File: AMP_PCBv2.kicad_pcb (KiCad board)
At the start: 2 copper layers, 2 parts, among them U1 Teensy4.0, U2 Logo

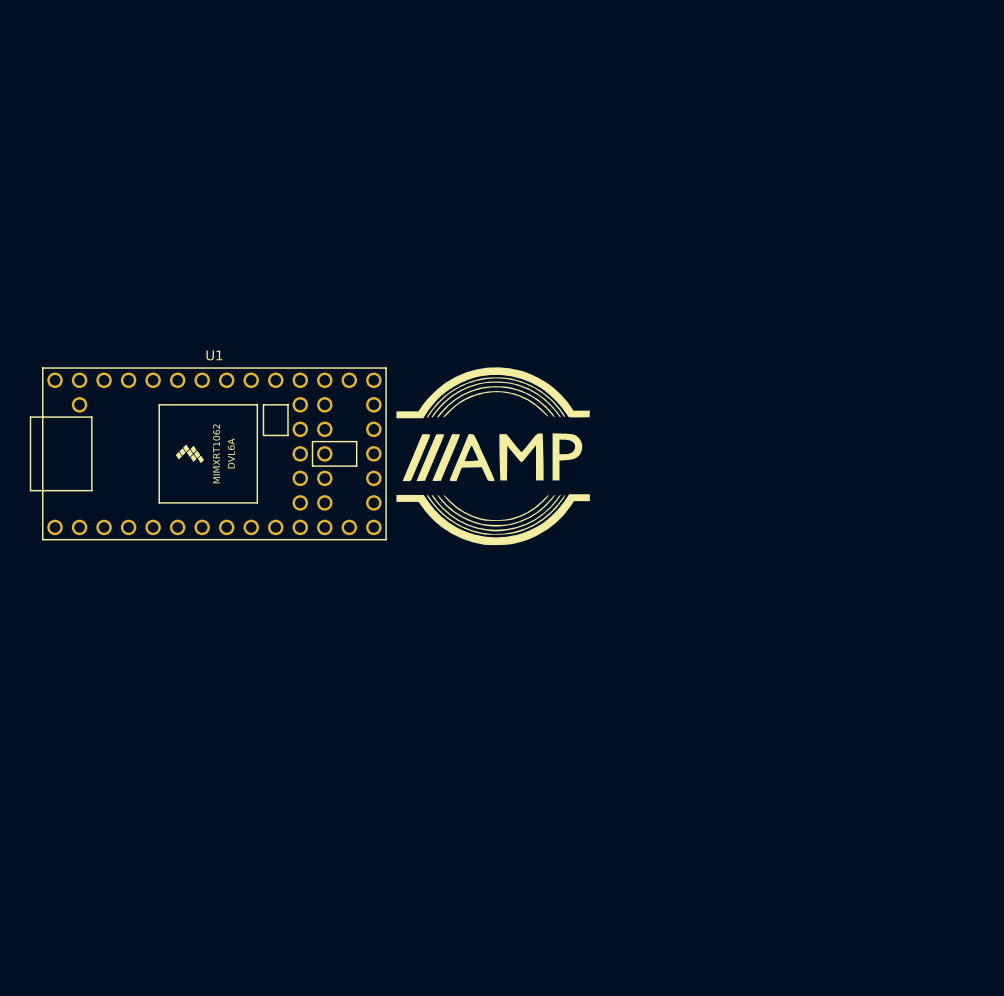
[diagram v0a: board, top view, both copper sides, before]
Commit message: Route PCB
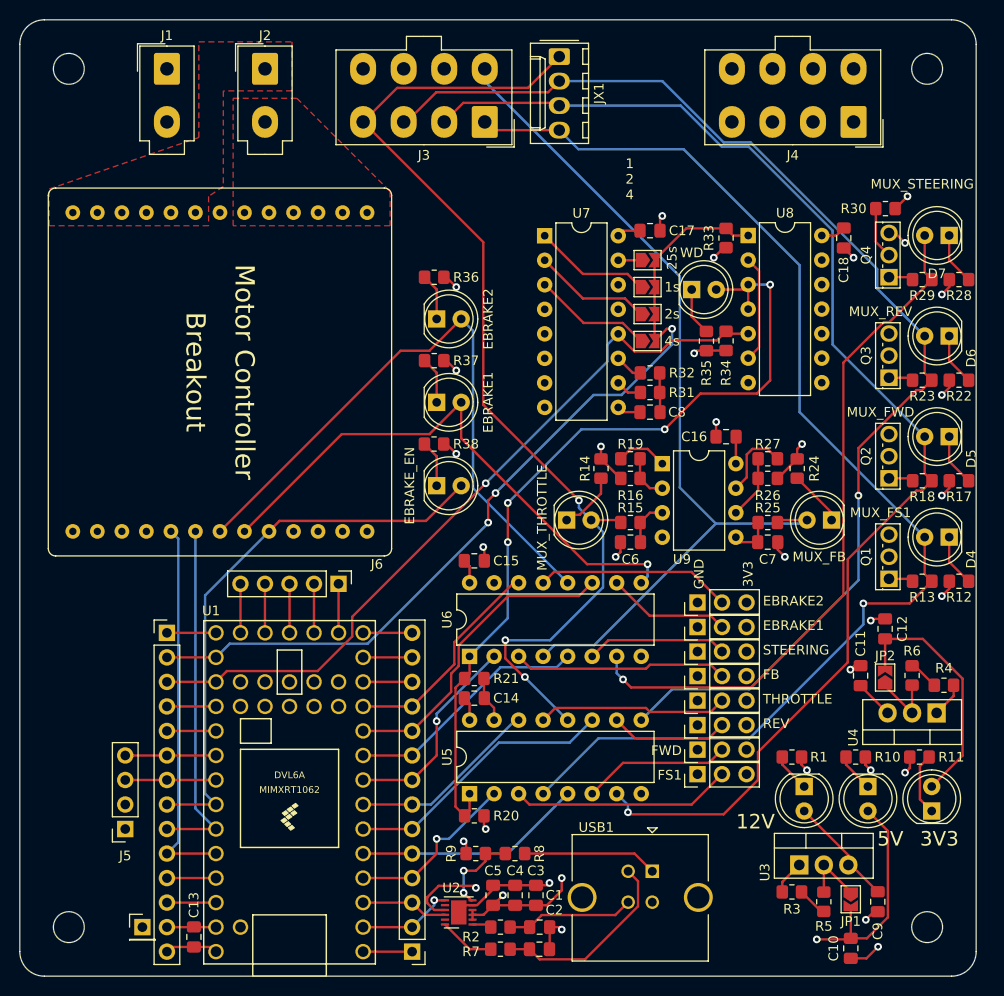
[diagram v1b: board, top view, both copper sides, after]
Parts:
- added C1: 47pF, Capacitor_SMD:C_0805_2012Metric_Pad1.18x1.45mm_HandSolder, F.Cu at (145.3, 134.6)
- added C10: 0.1uF, Capacitor_SMD:C_0805_2012Metric_Pad1.18x1.45mm_HandSolder, F.Cu at (177.5, 136.8)
- added C11: 0.1uF, Capacitor_SMD:C_0805_2012Metric_Pad1.18x1.45mm_HandSolder, F.Cu at (178.5, 108.6)
- added C12: 0.1uF, Capacitor_SMD:C_0805_2012Metric_Pad1.18x1.45mm_HandSolder, F.Cu at (181.1, 103.7)
- added C13: 0.1uF, Capacitor_SMD:C_0805_2012Metric_Pad1.18x1.45mm_HandSolder, F.Cu at (109.5, 135.6)
- added C14: 0.1uF, Capacitor_SMD:C_0805_2012Metric_Pad1.18x1.45mm_HandSolder, F.Cu at (138.5, 110.9)
- added C15: 0.1uF, Capacitor_SMD:C_0805_2012Metric_Pad1.18x1.45mm_HandSolder, F.Cu at (138.5, 96.7)
- added C16: 0.1uF, Capacitor_SMD:C_0805_2012Metric_Pad1.18x1.45mm_HandSolder, F.Cu at (164.6, 83.8)
- added C17: 0.1uF, Capacitor_SMD:C_0805_2012Metric_Pad1.18x1.45mm_HandSolder, F.Cu at (156.7, 62.5)
- added C18: 0.1uF, Capacitor_SMD:C_0805_2012Metric_Pad1.18x1.45mm_HandSolder, F.Cu at (176.8, 63.2)
- added C2: 47pF, Capacitor_SMD:C_0805_2012Metric_Pad1.18x1.45mm_HandSolder, F.Cu at (145.3, 136.9)
- added C3: 4.7uF, Capacitor_SMD:C_0805_2012Metric_Pad1.18x1.45mm_HandSolder, F.Cu at (144.9, 131.3)
- added C4: 100nF, Capacitor_SMD:C_0805_2012Metric_Pad1.18x1.45mm_HandSolder, F.Cu at (142.7, 131.3)
- added C5: 100nF, Capacitor_SMD:C_0805_2012Metric_Pad1.18x1.45mm_HandSolder, F.Cu at (140.5, 131.3)
- added C6: 10uF, Capacitor_SMD:C_0805_2012Metric_Pad1.18x1.45mm_HandSolder, F.Cu at (154.7, 94.7)
- added C7: 10uF, Capacitor_SMD:C_0805_2012Metric_Pad1.18x1.45mm_HandSolder, F.Cu at (168.9, 94.7)
- added C8: 10nF, Capacitor_SMD:C_0805_2012Metric_Pad1.18x1.45mm_HandSolder, F.Cu at (156.7, 81.3)
- added C9: 0.1uF, Capacitor_SMD:C_0805_2012Metric_Pad1.18x1.45mm_HandSolder, F.Cu at (180.3, 132.0)
- added D1: GN, LED_THT:LED_D5.0mm, F.Cu at (172.7, 120.1)
- added D10: YL, LED_THT:LED_D5.0mm, F.Cu at (134.6, 88.9)
- added D11: RD, LED_THT:LED_D5.0mm, F.Cu at (134.6, 80.3)
- added D12: RD, LED_THT:LED_D5.0mm, F.Cu at (134.6, 71.6)
- added D13: RD, LED_THT:LED_D5.0mm, F.Cu at (161.0, 68.6)
- added D2: GN, LED_THT:LED_D5.0mm, F.Cu at (179.3, 120.1)
- added D3: GN, LED_THT:LED_D5.0mm, F.Cu at (185.9, 122.6)
- added D4: YL, LED_THT:LED_D5.0mm, F.Cu at (187.7, 94.2)
- added D5: YL, LED_THT:LED_D5.0mm, F.Cu at (187.7, 83.8)
- added D6: YL, LED_THT:LED_D5.0mm, F.Cu at (187.7, 73.4)
- added D7: YL, LED_THT:LED_D5.0mm, F.Cu at (187.7, 63.0)
- added D8: YL, LED_THT:LED_D5.0mm, F.Cu at (148.1, 92.5)
- added D9: YL, LED_THT:LED_D5.0mm, F.Cu at (175.5, 92.5)
- added J1: POWER, Connector_Molex:Molex_Mini-Fit_Jr_5566-02A_2x01_P4.20mm_Vertical, F.Cu at (106.7, 45.7)
- added J2: EBRAKE, Connector_Molex:Molex_Mini-Fit_Jr_5566-02A_2x01_P4.20mm_Vertical, F.Cu at (116.8, 45.7)
- added J3: MC, Connector_Molex:Molex_Mini-Fit_Jr_5566-08A_2x04_P4.20mm_Vertical, F.Cu at (139.6, 51.2)
- added J4: STEERING, Connector_Molex:Molex_Mini-Fit_Jr_5566-08A_2x04_P4.20mm_Vertical, F.Cu at (177.8, 51.2)
- added J5: OLED Breakout, Connector_PinSocket_2.54mm:PinSocket_1x04_P2.54mm_Vertical, F.Cu at (102.4, 124.5)
- added J6: EBRAKE_BREAKOUT, AMP:AMP_Brake_Controller_Breakout, F.Cu at (130.0, 96.2)
- added JP1: 5VOB, Jumper:SolderJumper-2_P1.3mm_Open_TrianglePad1.0x1.5mm, F.Cu at (177.5, 131.7)
- added JP10: Jumper_EBRAKE2, Connector_PinHeader_2.54mm:PinHeader_1x03_P2.54mm_Vertical, F.Cu at (161.6, 101.0)
- added JP11: 0.25s, Jumper:SolderJumper-2_P1.3mm_Open_TrianglePad1.0x1.5mm, F.Cu at (156.5, 65.5)
- added JP12: 1s, Jumper:SolderJumper-2_P1.3mm_Open_TrianglePad1.0x1.5mm, F.Cu at (156.5, 68.3)
- added JP13: 2s, Jumper:SolderJumper-2_P1.3mm_Open_TrianglePad1.0x1.5mm, F.Cu at (156.5, 71.1)
- added JP14: 4s, Jumper:SolderJumper-2_P1.3mm_Open_TrianglePad1.0x1.5mm, F.Cu at (156.5, 73.9)
- added JP2: 3V3OB, Jumper:SolderJumper-2_P1.3mm_Open_TrianglePad1.0x1.5mm, F.Cu at (181.1, 108.8)
- added JP3: Jumper_FS1, Connector_PinHeader_2.54mm:PinHeader_1x03_P2.54mm_Vertical, F.Cu at (161.6, 118.8)
- added JP4: Jumper_FWD, Connector_PinHeader_2.54mm:PinHeader_1x03_P2.54mm_Vertical, F.Cu at (161.6, 116.2)
- added JP5: Jumper_REV, Connector_PinHeader_2.54mm:PinHeader_1x03_P2.54mm_Vertical, F.Cu at (161.6, 113.7)
- added JP6: Jumper_THROTTLE, Connector_PinHeader_2.54mm:PinHeader_1x03_P2.54mm_Vertical, F.Cu at (161.6, 111.2)
- added JP7: Jumper_RB, Connector_PinHeader_2.54mm:PinHeader_1x03_P2.54mm_Vertical, F.Cu at (161.6, 108.6)
- added JP8: Jumper_STEERING, Connector_PinHeader_2.54mm:PinHeader_1x03_P2.54mm_Vertical, F.Cu at (161.6, 106.1)
- added JP9: Jumper_EBRAKE1, Connector_PinHeader_2.54mm:PinHeader_1x03_P2.54mm_Vertical, F.Cu at (161.6, 103.5)
- added JT1: Conn_01x14_Male, Connector_PinHeader_2.54mm:PinHeader_1x14_P2.54mm_Vertical, F.Cu at (132.1, 137.2)
- added JT2: Conn_01x05_Male, Connector_PinHeader_2.54mm:PinHeader_1x05_P2.54mm_Vertical, F.Cu at (124.5, 99.1)
- added JT3: Conn_01x14_Male, Connector_PinHeader_2.54mm:PinHeader_1x14_P2.54mm_Vertical, F.Cu at (106.7, 104.1)
- added JT4: Conn_01x01_Male, Connector_PinHeader_2.54mm:PinHeader_1x01_P2.54mm_Vertical, F.Cu at (104.1, 134.6)
- added JX1: MC_OLD, Connector_Molex:Molex_KK-254_AE-6410-04A_1x04_P2.54mm_Vertical, F.Cu at (147.3, 44.5)
- added Q1: Q_NMOS_GDS, Package_TO_SOT_THT:TO-251-3_Vertical, F.Cu at (181.5, 98.5)
- added Q2: Q_NMOS_GDS, Package_TO_SOT_THT:TO-251-3_Vertical, F.Cu at (181.5, 88.1)
- added Q3: Q_NMOS_GDS, Package_TO_SOT_THT:TO-251-3_Vertical, F.Cu at (181.5, 77.7)
- added Q4: Q_NMOS_GDS, Package_TO_SOT_THT:TO-251-3_Vertical, F.Cu at (181.5, 67.3)
- added R1: 560, Resistor_SMD:R_0805_2012Metric_Pad1.20x1.40mm_HandSolder, F.Cu at (171.4, 117.0)
- added R10: 130, Resistor_SMD:R_0805_2012Metric_Pad1.20x1.40mm_HandSolder, F.Cu at (178.0, 117.0)
- added R11: 56, Resistor_SMD:R_0805_2012Metric_Pad1.20x1.40mm_HandSolder, F.Cu at (184.6, 117.0)
- added R12: 56, Resistor_SMD:R_0805_2012Metric_Pad1.20x1.40mm_HandSolder, F.Cu at (188.7, 98.8)
- added R13: 1K, Resistor_SMD:R_0805_2012Metric_Pad1.20x1.40mm_HandSolder, F.Cu at (184.9, 98.8)
- added R14: 56, Resistor_SMD:R_0805_2012Metric_Pad1.20x1.40mm_HandSolder, F.Cu at (151.6, 87.1)
- added R15: 1K, Resistor_SMD:R_0805_2012Metric_Pad1.20x1.40mm_HandSolder, F.Cu at (154.7, 92.7)
- added R16: 1K, Resistor_SMD:R_0805_2012Metric_Pad1.20x1.40mm_HandSolder, F.Cu at (154.7, 88.1)
- added R17: 56, Resistor_SMD:R_0805_2012Metric_Pad1.20x1.40mm_HandSolder, F.Cu at (188.7, 88.4)
- added R18: 1K, Resistor_SMD:R_0805_2012Metric_Pad1.20x1.40mm_HandSolder, F.Cu at (184.9, 88.4)
- added R19: 1.8K, Resistor_SMD:R_0805_2012Metric_Pad1.20x1.40mm_HandSolder, F.Cu at (154.7, 86.1)
- added R2: 27, Resistor_SMD:R_0805_2012Metric_Pad1.20x1.40mm_HandSolder, F.Cu at (141.2, 134.6)
- added R20: 10K, Resistor_SMD:R_0805_2012Metric_Pad1.20x1.40mm_HandSolder, F.Cu at (138.5, 123.1)
- added R21: 10K, Resistor_SMD:R_0805_2012Metric_Pad1.20x1.40mm_HandSolder, F.Cu at (138.5, 108.9)
- added R22: 56, Resistor_SMD:R_0805_2012Metric_Pad1.20x1.40mm_HandSolder, F.Cu at (188.7, 78.0)
- added R23: 1K, Resistor_SMD:R_0805_2012Metric_Pad1.20x1.40mm_HandSolder, F.Cu at (184.9, 78.0)
- added R24: 56, Resistor_SMD:R_0805_2012Metric_Pad1.20x1.40mm_HandSolder, F.Cu at (172.0, 87.1)
- added R25: 1K, Resistor_SMD:R_0805_2012Metric_Pad1.20x1.40mm_HandSolder, F.Cu at (168.9, 92.7)
- added R26: 1K, Resistor_SMD:R_0805_2012Metric_Pad1.20x1.40mm_HandSolder, F.Cu at (168.9, 88.1)
- added R27: 1.8K, Resistor_SMD:R_0805_2012Metric_Pad1.20x1.40mm_HandSolder, F.Cu at (168.9, 86.1)
- added R28: 56, Resistor_SMD:R_0805_2012Metric_Pad1.20x1.40mm_HandSolder, F.Cu at (188.7, 67.5)
- added R29: 1K, Resistor_SMD:R_0805_2012Metric_Pad1.20x1.40mm_HandSolder, F.Cu at (184.9, 67.5)
- added R3: 10K, Resistor_SMD:R_0805_2012Metric_Pad1.20x1.40mm_HandSolder, F.Cu at (171.4, 131.0)
- added R30: 1K, Resistor_SMD:R_0805_2012Metric_Pad1.20x1.40mm_HandSolder, F.Cu at (181.1, 60.2)
- added R31: 15K, Resistor_SMD:R_0805_2012Metric_Pad1.20x1.40mm_HandSolder, F.Cu at (156.7, 79.2)
- added R32: 6.2K, Resistor_SMD:R_0805_2012Metric_Pad1.20x1.40mm_HandSolder, F.Cu at (156.7, 77.2)
- added R33: 10K, Resistor_SMD:R_0805_2012Metric_Pad1.20x1.40mm_HandSolder, F.Cu at (164.6, 63.2)
- added R34: 10K, Resistor_SMD:R_0805_2012Metric_Pad1.20x1.40mm_HandSolder, F.Cu at (164.6, 73.9)
- added R35: 33, Resistor_SMD:R_0805_2012Metric_Pad1.20x1.40mm_HandSolder, F.Cu at (162.6, 73.9)
- added R36: 33, Resistor_SMD:R_0805_2012Metric_Pad1.20x1.40mm_HandSolder, F.Cu at (134.4, 67.3)
- added R37: 33, Resistor_SMD:R_0805_2012Metric_Pad1.20x1.40mm_HandSolder, F.Cu at (134.4, 75.9)
- added R38: 56, Resistor_SMD:R_0805_2012Metric_Pad1.20x1.40mm_HandSolder, F.Cu at (134.3, 84.6)
- added R4: 10K, Resistor_SMD:R_0805_2012Metric_Pad1.20x1.40mm_HandSolder, F.Cu at (187.2, 109.6)
- added R5: 3.3K, Resistor_SMD:R_0805_2012Metric_Pad1.20x1.40mm_HandSolder, F.Cu at (174.7, 132.0)
- added R6: 6.2K, Resistor_SMD:R_0805_2012Metric_Pad1.20x1.40mm_HandSolder, F.Cu at (183.9, 108.6)
- added R7: 27, Resistor_SMD:R_0805_2012Metric_Pad1.20x1.40mm_HandSolder, F.Cu at (141.2, 136.9)
- added R8: 4.7K, Resistor_SMD:R_0805_2012Metric_Pad1.20x1.40mm_HandSolder, F.Cu at (142.7, 127.0)
- added R9: 10K, Resistor_SMD:R_0805_2012Metric_Pad1.20x1.40mm_HandSolder, F.Cu at (138.7, 127.0)
- added REF**: MountingHole_3.2mm_M3, MountingHole:MountingHole_3.2mm_M3, F.Cu at (96.5, 45.7)
- added REF**: MountingHole_3.2mm_M3, MountingHole:MountingHole_3.2mm_M3, F.Cu at (96.5, 134.6)
- added REF**: MountingHole_3.2mm_M3, MountingHole:MountingHole_3.2mm_M3, F.Cu at (185.4, 45.7)
- added REF**: MountingHole_3.2mm_M3, MountingHole:MountingHole_3.2mm_M3, F.Cu at (185.4, 134.6)
- added U3: LM1117-ADJ, Package_TO_SOT_THT:TO-220-3_Vertical, F.Cu at (172.2, 128.2)
- added U4: LM1117-ADJ, Package_TO_SOT_THT:TO-220-3_Vertical, F.Cu at (186.4, 112.4)
- added U5: 74HC157, Package_DIP:DIP-16_W7.62mm, F.Cu at (138.0, 120.8)
- added U6: 74HC157, Package_DIP:DIP-16_W7.62mm, F.Cu at (138.0, 106.6)
- added U7: 74HC4060, Package_DIP:DIP-16_W7.62mm, F.Cu at (145.8, 63.0)
- added U8: 74HC00, Package_DIP:DIP-14_W7.62mm, F.Cu at (166.9, 63.0)
- added U9: TLV272, Package_DIP:DIP-8_W7.62mm, F.Cu at (158.0, 86.6)
- added USB1: USB_B, Connector_USB:USB_B_TE_5787834_Vertical, F.Cu at (157.0, 128.8)
- U2: value Logo -> FT234XD; footprint AMP:Logo -> Package_DFN_QFN:DFN-12-1EP_3x3mm_P0.5mm_EP1.6x2.5mm
- moved U2 47.2 mm to (136.9, 133.1), turned to 180 degrees
- moved U1 35.9 mm to (119.4, 120.7), turned to 90 degrees
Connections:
- U1 pad 1: unconnected-(U1-Pad1) -> GND
- U1 pad 10: unconnected-(U1-Pad10) -> /MCU_EBRAKE1
- U1 pad 11: unconnected-(U1-Pad11) -> /MCU_EBRAKE2
- U1 pad 12: unconnected-(U1-Pad12) -> Net-(U1-Pad12)
- U1 pad 13: unconnected-(U1-Pad13) -> Net-(U1-Pad13)
- U1 pad 14: unconnected-(U1-Pad14) -> Net-(U1-Pad14)
- U1 pad 15: unconnected-(U1-Pad15) -> Net-(U1-Pad15)
- U1 pad 16: unconnected-(U1-Pad16) -> Net-(U1-Pad16)
- U1 pad 17: unconnected-(U1-Pad17) -> GND
- U1 pad 18: unconnected-(U1-Pad18) -> Net-(U1-Pad18)
- U1 pad 19: unconnected-(U1-Pad19) -> Net-(U1-Pad19)
- U1 pad 2: unconnected-(U1-Pad2) -> /RX1
- U1 pad 20: unconnected-(U1-Pad20) -> Net-(U1-Pad20)
- U1 pad 21: unconnected-(U1-Pad21) -> /WD_SET
- U1 pad 22: unconnected-(U1-Pad22) -> /WD_RESET
- U1 pad 23: unconnected-(U1-Pad23) -> Net-(U1-Pad23)
- U1 pad 24: unconnected-(U1-Pad24) -> Net-(U1-Pad24)
- U1 pad 25: unconnected-(U1-Pad25) -> /OLED_SDA
- U1 pad 26: unconnected-(U1-Pad26) -> /OLED_SCL
- U1 pad 27: unconnected-(U1-Pad27) -> /EBRAKE_EN
- U1 pad 28: unconnected-(U1-Pad28) -> /EBRAKE_IS1
- U1 pad 29: unconnected-(U1-Pad29) -> /EBRAKE_IS2
- U1 pad 3: unconnected-(U1-Pad3) -> /TX1
- U1 pad 30: unconnected-(U1-Pad30) -> Net-(U1-Pad30)
- U1 pad 31: unconnected-(U1-Pad31) -> Net-(U1-Pad31)
- U1 pad 32: unconnected-(U1-Pad32) -> GND
- U1 pad 33: unconnected-(U1-Pad33) -> +5V
- U1 pad 34: unconnected-(U1-Pad34) -> Net-(U1-Pad34)
- U1 pad 4: unconnected-(U1-Pad4) -> /MCU_FS1
- U1 pad 5: unconnected-(U1-Pad5) -> /MCU_FWD
- U1 pad 6: unconnected-(U1-Pad6) -> /MCU_REV
- U1 pad 7: unconnected-(U1-Pad7) -> /MCU_THROTTLE
- U1 pad 8: unconnected-(U1-Pad8) -> /MCU_FB
- U1 pad 9: unconnected-(U1-Pad9) -> /MCU_STEERING
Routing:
- net +5V: track 0.00 -> 201.0 mm, vias 0 -> 1
- net /MUX_FWD: track 0.00 -> 132.9 mm, vias 0 -> 1
- net /MUX_FS1: track 0.00 -> 127.8 mm, vias 0 -> 1
- net /MUX_REV: track 0.00 -> 125.4 mm, vias 0 -> 1
- net +3V3: track 0.00 -> 115.2 mm, vias 0 -> 3
- net /MUX_THROTTLE: track 0.00 -> 108.2 mm, vias 0 -> 3
- net GND: track 0.00 -> 95.4 mm, vias 0 -> 29
- net /MUX_FB: track 0.00 -> 93.4 mm
- net /WD_SET: track 0.00 -> 90.8 mm, vias 0 -> 3
- net /WD_SEL: track 0.00 -> 88.3 mm, vias 0 -> 4
- net /WD_RESET: track 0.00 -> 79.2 mm, vias 0 -> 1
- net /MUX_STEERING: track 0.00 -> 71.5 mm, vias 0 -> 1
- net /MUX_EBRAKE2: track 0.00 -> 66.0 mm
- net /MUX_EBRAKE1: track 0.00 -> 58.6 mm, vias 0 -> 1
- net /EBRAKE_EN: track 0.00 -> 58.4 mm
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- added copper zone on In1.Cu, net +12V
- added copper zone on F.Cu, net /OUT_EBRAKE1
- added copper zone on F.Cu, net /OUT_EBRAKE2
- added copper zone on In2.Cu, net GND
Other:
- board outline added: 99.1 x 99.1 mm
- copper layers 2 -> 4
- board text added: ".25s"
- board text added: "1 2 4"
- board text added: "12V"
- board text added: "1s"
- board text added: "2s"
- board text added: "3V3"
- board text added: "4s"
- board text added: "5V"
- board text added: "EBRAKE1"
- board text added: "EBRAKE2"
- board text added: "EBRAKE_EN"
- board text added: "FB"
- board text added: "FS1"
- board text added: "FWD"
- board text added: "GND"
- board text added: "MUX_FB"
- board text added: "MUX_FS1"
- board text added: "MUX_FWD"
- board text added: "MUX_REV"
- board text added: "MUX_STEERING"
- board text added: "MUX_THROTTLE"
- board text added: "REV"
- board text added: "STEERING"
- board text added: "THROTTLE"
- board text added: "WD"
